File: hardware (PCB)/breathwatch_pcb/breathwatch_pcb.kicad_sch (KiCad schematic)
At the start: 8 parts, among them J1 Conn_01x08_Socket, J2 Conn_01x08_Socket, J4 Conn_01x08_Socket, J5 USB_C_Receptacle_PowerOnly_6P, Q1 AO3401A, SW1 SW_Push

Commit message: added a bit to code
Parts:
- R1, R2: footprint Resistor_THT:R_Axial_DIN0207_L6.3mm_D2.5mm_P7.62mm_Horizontal -> Resistor_SMD:R_0603_1608Metric
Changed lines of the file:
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@@
 			)
 		)
-		(property "Footprint" "Resistor_THT:R_Axial_DIN0207_L6.3mm_D2.5mm_P7.62mm_Horizontal"
+		(property "Footprint" "Resistor_SMD:R_0603_1608Metric"
 			(at 89.662 85.09 90)
 			(effects
@@
 			)
 		)
-		(property "Footprint" "Resistor_THT:R_Axial_DIN0207_L6.3mm_D2.5mm_P7.62mm_Horizontal"
+		(property "Footprint" "Resistor_SMD:R_0603_1608Metric"
 			(at 94.742 96.52 90)
 			(effects

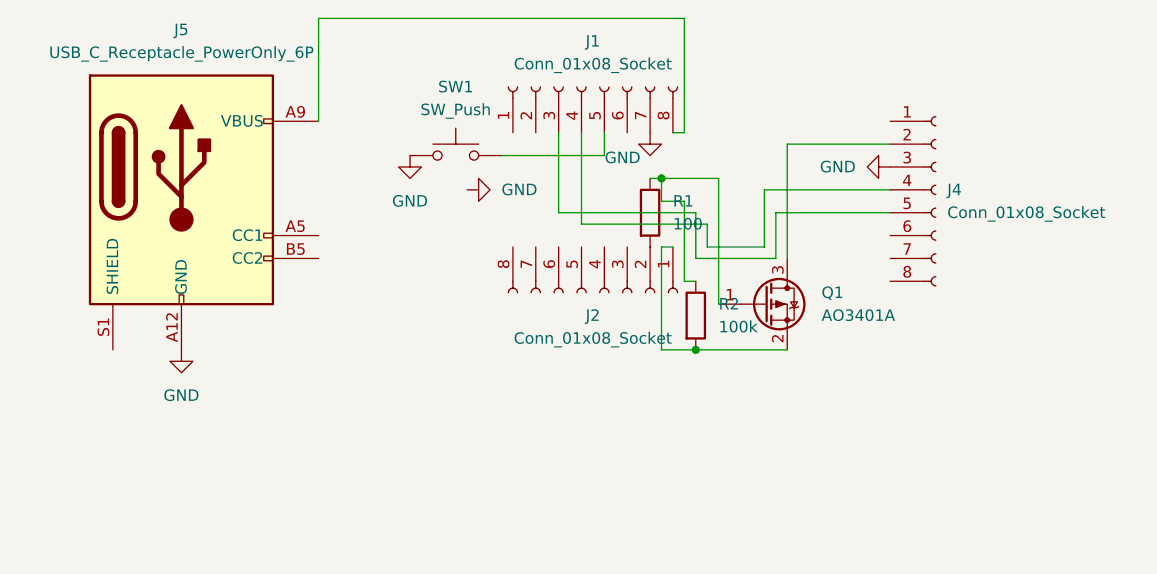
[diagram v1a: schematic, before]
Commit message: PCB Design
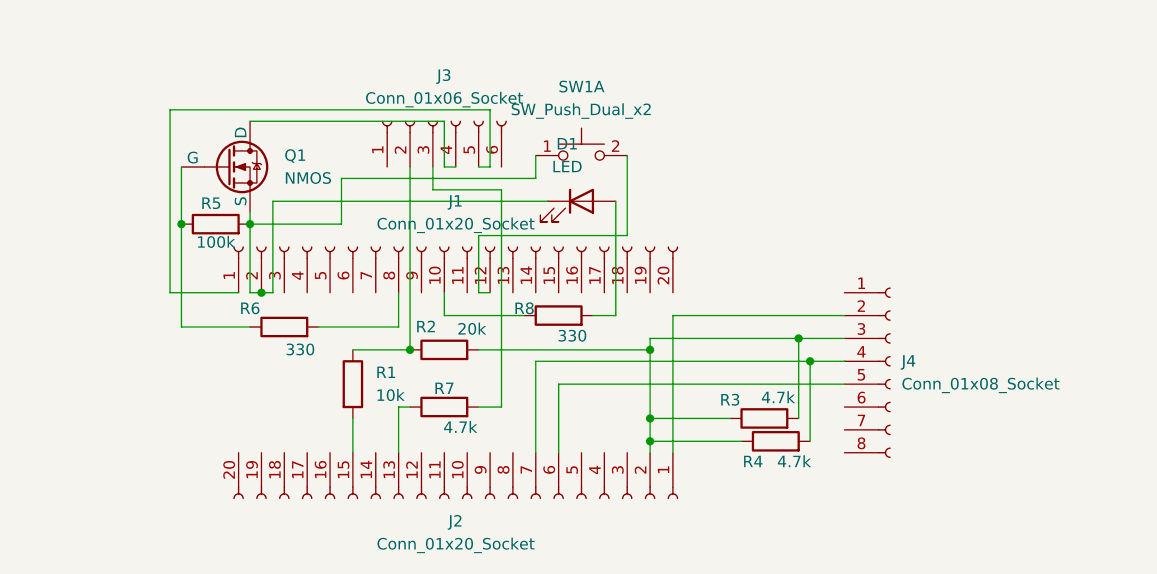
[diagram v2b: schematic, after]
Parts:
- removed J1: Conn_01x08_Socket, Connector_PinSocket_2.54mm:PinSocket_1x08_P2.54mm_Vertical_SMD_Pin1Left, symbol Connector:Conn_01x08_Socket
- removed J2: Conn_01x08_Socket, Connector_PinSocket_2.54mm:PinSocket_1x08_P2.54mm_Vertical_SMD_Pin1Right, symbol Connector:Conn_01x08_Socket
- removed J5: USB_C_Receptacle_PowerOnly_6P, Connector_USB:USB_C_Receptacle_GCT_USB4125-xx-x_6P_TopMnt_Horizontal, symbol Connector:USB_C_Receptacle_PowerOnly_6P
- removed Q1: AO3401A, Package_TO_SOT_SMD:SOT-23, symbol Transistor_FET:AO3401A
- removed SW1: SW_Push, Button_Switch_THT:SW_PUSH_6mm_H7.3mm, symbol Switch:SW_Push
- added D1: LED, LED_THT:LED_D5.0mm, symbol Device:LED
- added J1, J2: Conn_01x20_Socket, Connector_PinSocket_2.54mm:PinSocket_1x20_P2.54mm_Vertical, symbol Connector:Conn_01x20_Socket
- added J3: Conn_01x06_Socket, Connector_PinSocket_2.54mm:PinSocket_1x06_P2.54mm_Vertical, symbol Connector:Conn_01x06_Socket
- added Q1: NMOS, Package_TO_SOT_THT:TO-220-3_Vertical, symbol Simulation_SPICE:NMOS
- added R3, R4, R7: 4.7k, Resistor_SMD:R_0815_2038Metric, symbol Device:R
- added R5: 100k, Resistor_SMD:R_0815_2038Metric, symbol Device:R
- added R6, R8: 330, Resistor_SMD:R_0815_2038Metric, symbol Device:R
- added SW1: SW_Push_Dual_x2, Button_Switch_THT:SW_PUSH_6mm_H4.3mm, symbol Switch:SW_Push_Dual_x2
- J4: footprint Connector_PinSocket_2.54mm:PinSocket_1x08_P2.54mm_Vertical_SMD_Pin1Right -> Connector_PinSocket_2.54mm:PinSocket_1x08_P2.54mm_Vertical
- R1: value 100 -> 10k; footprint Resistor_SMD:R_0603_1608Metric -> Resistor_SMD:R_0815_2038Metric
- R2: value 100k -> 20k; footprint Resistor_SMD:R_0603_1608Metric -> Resistor_SMD:R_0815_2038Metric
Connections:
- net GND is gone; now on an unnamed net: J4.3 (Pin_3)
- net at J4.5 (Pin_5): now also J2.6 (Pin_6)
- net at J4.4 (Pin_4): now also J2.7 (Pin_7), R4.2
- net at J4.2 (Pin_2): now also J2.1 (Pin_1)
- net at R1.1, R2.1: now also J3.2 (Pin_2)
- net at R2.2: now also J2.2 (Pin_2), R3.1, R3.2, R4.1
- net at R1.2: now also J2.15 (Pin_15)
- new net: D1.1 (K), J1.2 (Pin_2), Q1.3 (S), R5.2, SW1.1 (C)
- new net: J1.12 (Pin_12), SW1.2 (D)
- new net: J3.4 (Pin_4), Q1.1 (D)
- new net: Q1.2 (G), R5.1, R6.1
- new net: J1.8 (Pin_8), R6.2
- new net: J1.10 (Pin_10), R8.1
- new net: D1.2 (A), R8.2
- new net: J2.13 (Pin_13), R7.1
- new net: J1.1 (Pin_1), J3.5 (Pin_5)
- new net: J3.3 (Pin_3), R7.2
